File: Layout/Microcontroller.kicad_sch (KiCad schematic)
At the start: 21 parts, among them IC1 OPT3101RHFR, J1 Conn_01x07_MountingPin, J2 Conn_01x07_Pin(Display), J3 USB_B_Micro, SW1 SW_Omron_B3FS, SW2 SW_Omron_B3FS, U2 STM32L4Q5CGTx, U6 USBLC6-2SC6

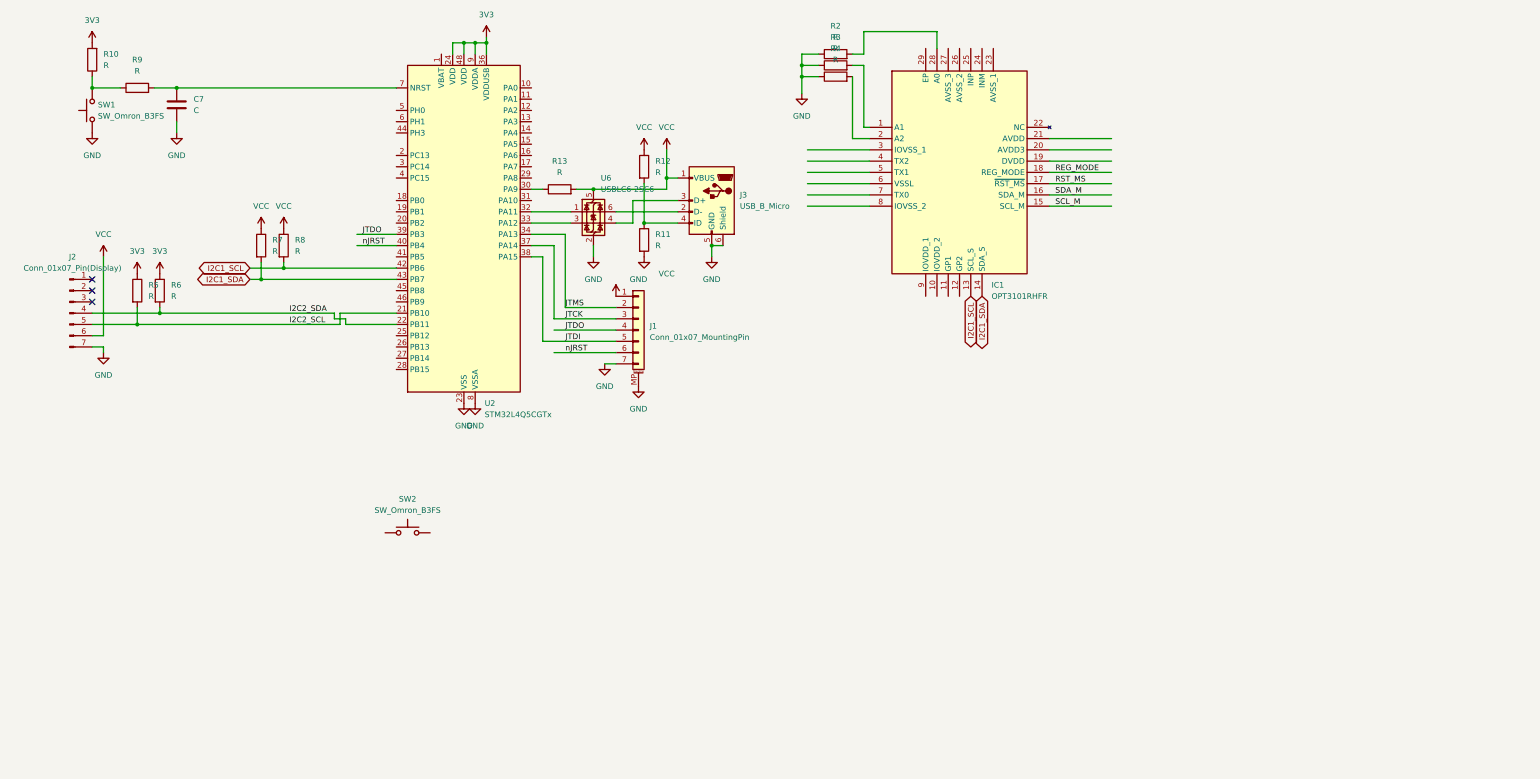
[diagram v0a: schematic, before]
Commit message: Layout merged together
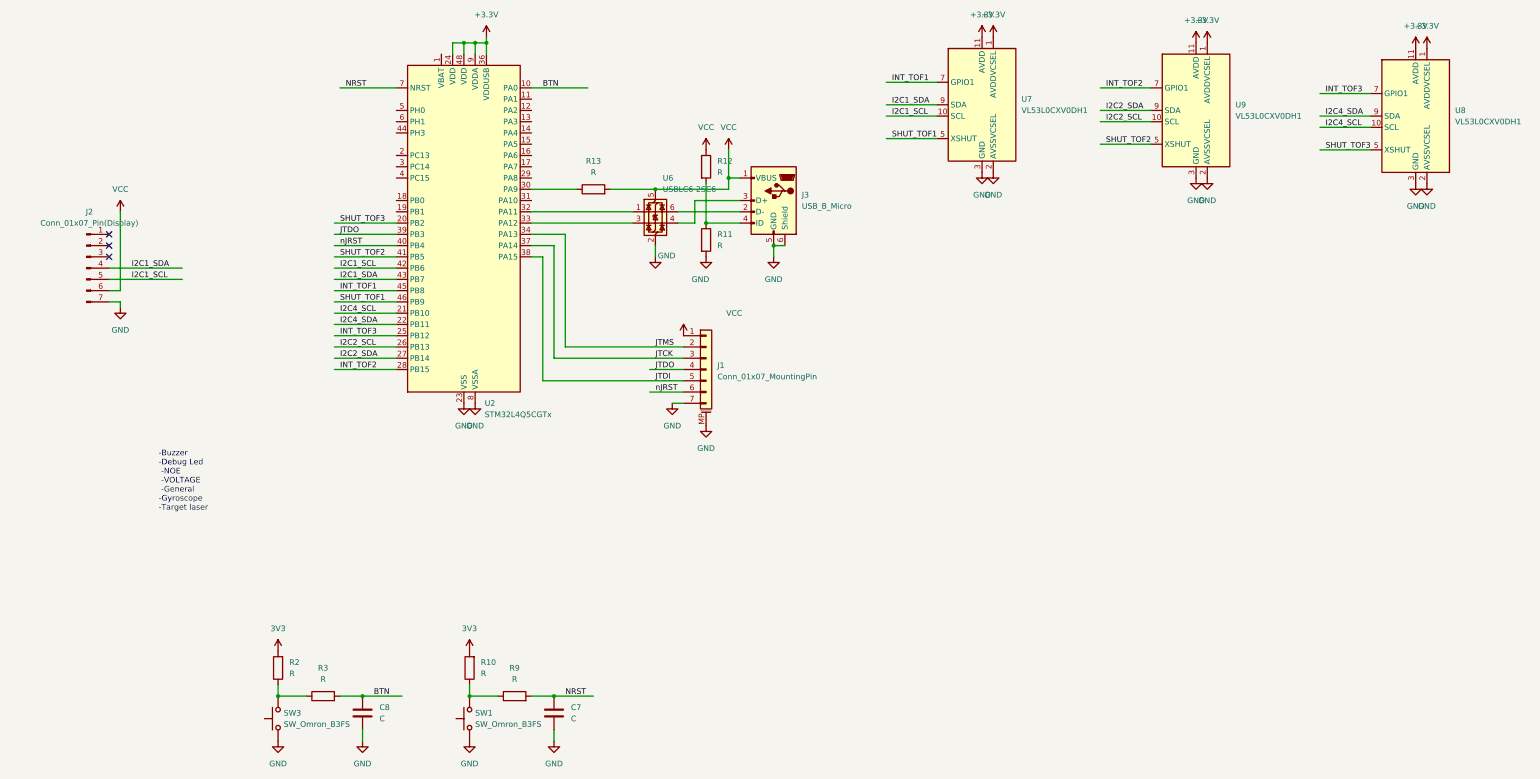
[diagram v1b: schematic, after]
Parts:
- removed IC1: OPT3101RHFR, ToF Driver:QFN50P400X500X100-29N-D, symbol OPT3101RHFR:OPT3101RHFR
- removed R4, R5, R6, R7, R8: R, symbol Device:R
- removed SW2: SW_Omron_B3FS, symbol Switch:SW_Omron_B3FS
- added C8: C, symbol Device:C
- added SW3: SW_Omron_B3FS, symbol Switch:SW_Omron_B3FS
- added U7, U8, U9: VL53L0CXV0DH1, Sensor_Distance:ST_VL53L1x, symbol Sensor_Distance:VL53L0CXV0DH1
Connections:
- net 3V3: now also R2.2; no longer U2.24 (VDD), U2.36 (VDDUSB), U2.48 (VDD), U2.9 (VDDA)
- net GND: now also C8.2, SW3.1, U7.12 (GND), U7.2 (AVSSVCSEL), U7.3 (GND), U7.4 (GND), U7.6 (GND), U8.12 (GND), U8.2 (AVSSVCSEL), U8.3 (GND), U8.4 (GND), U8.6 (GND), U9.12 (GND), U9.2 (AVSSVCSEL), U9.3 (GND), U9.4 (GND), U9.6 (GND); no longer R2.1, R3.1
- net I2C1_SCL: now also J2.5 (Pin_5), U7.10 (SCL)
- net I2C1_SDA: now also J2.4 (Pin_4), U7.9 (SDA)
- net I2C2_SCL: now also U2.26 (PB13), U9.10 (SCL); no longer J2.5 (Pin_5), U2.21 (PB10)
- net I2C2_SDA: now also U2.27 (PB14), U9.9 (SDA); no longer J2.4 (Pin_4), U2.22 (PB11)
- net BTN: now reaches R3.2
- net BTN: now also U2.10 (PA0), C8.1
- net SHUT_TOF3: now reaches U2.20 (PB2)
- net SHUT_TOF3: now also U8.5 (XSHUT)
- net INT_TOF3: now reaches U2.25 (PB12)
- net INT_TOF3: now also U8.7 (GPIO1)
- net INT_TOF2: now reaches U2.28 (PB15)
- net INT_TOF2: now also U9.7 (GPIO1)
- net SHUT_TOF2: now reaches U2.41 (PB5)
- net SHUT_TOF2: now also U9.5 (XSHUT)
- net INT_TOF1: now reaches U2.45 (PB8)
- net INT_TOF1: now also U7.7 (GPIO1)
- net SHUT_TOF1: now reaches U2.46 (PB9)
- net SHUT_TOF1: now also U7.5 (XSHUT)
- net NRST: now reaches C7.1, R9.2, U2.7 (NRST)
- new net: R2.1, R3.1, SW3.2
- new net +3.3V: U2.24 (VDD), U2.36 (VDDUSB), U2.48 (VDD), U2.9 (VDDA), U7.1 (AVDDVCSEL), U7.11 (AVDD), U8.1 (AVDDVCSEL), U8.11 (AVDD), U9.1 (AVDDVCSEL), U9.11 (AVDD)
- new net I2C4_SCL: U2.21 (PB10), U8.10 (SCL)
- new net I2C4_SDA: U2.22 (PB11), U8.9 (SDA)
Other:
- note added: "-Buzzer -Debug Led -NOE -VOLTAGE -General -Gyroscope -Target laser"
- moved on the sheet: C7, J1, J2, J3, R10, R11, R12, R13, R9, SW1, U6
